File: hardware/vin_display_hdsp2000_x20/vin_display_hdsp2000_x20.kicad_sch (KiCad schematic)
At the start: 56 parts, among them J1 DEBUG, J2 USB_B_Micro, J3 DEBUG_UART, J4 IF_UART, J5 AUX_CONNECTOR, J6 Conn_01x02, Q1 BSS138, Q7 DMG2301L, SW1 SW_RESET, SW2 BOOTSEL, SW3 KNOB, U1 W25Q16JVSNIQ, U2 MIC23050-SYML, U3 RP2040, X1 12MHz

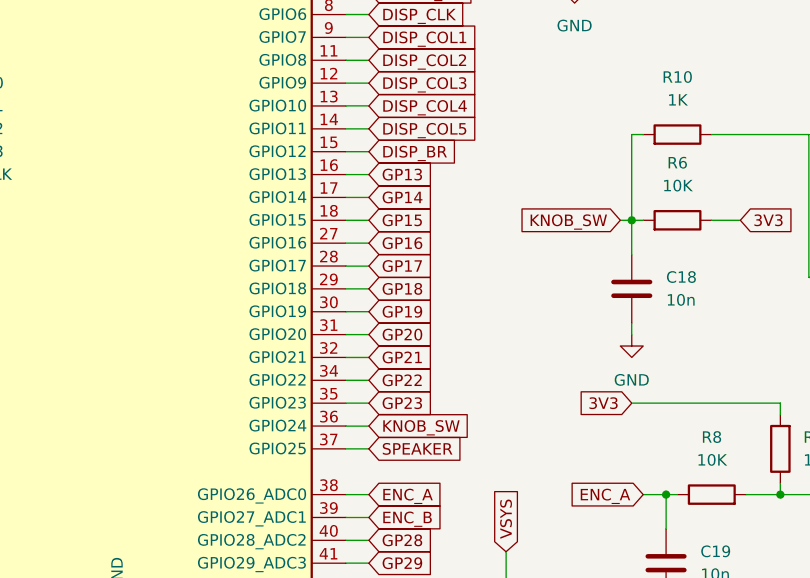
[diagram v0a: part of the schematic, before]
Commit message: hdsp2000_x20 minor changes
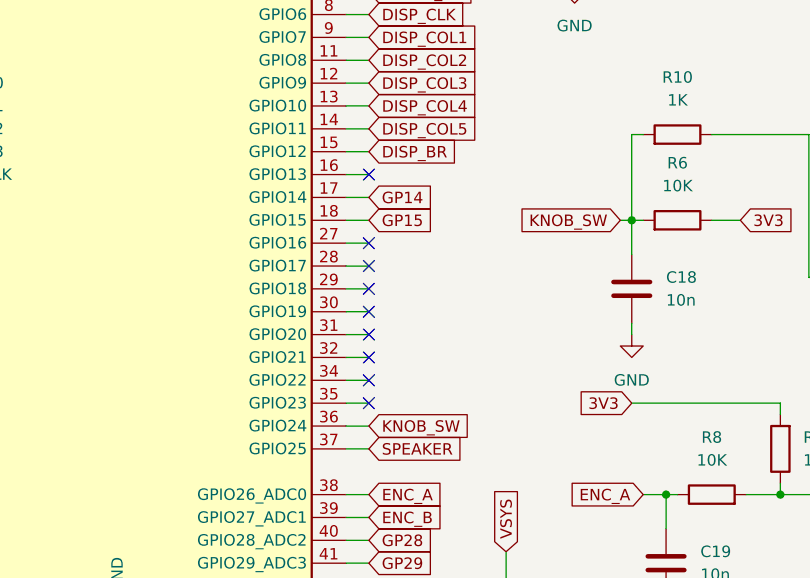
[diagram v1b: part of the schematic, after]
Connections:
- net GP13: no longer names the net of U3.16 (GPIO13)
- net GP16: no longer names the net of U3.27 (GPIO16)
- net GP17: no longer names the net of U3.28 (GPIO17)
- net GP18: no longer names the net of U3.29 (GPIO18)
- net GP19: no longer names the net of U3.30 (GPIO19)
- net GP20: no longer names the net of U3.31 (GPIO20)
- net GP21: no longer names the net of U3.32 (GPIO21)
- net GP22: no longer names the net of U3.34 (GPIO22)
- net GP23: no longer names the net of U3.35 (GPIO23)
- no-connect marks 1 -> 10
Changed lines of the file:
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@@
   (junction (at 130.81 22.86) (diameter 0) (color 0 0 0 0)
   )
+  (no_connect (at 181.61 97.79))
+  (no_connect (at 181.61 90.17))
+  (no_connect (at 181.61 92.71))
+  (no_connect (at 181.61 82.55))
+  (no_connect (at 181.61 95.25))
+  (no_connect (at 181.61 102.87))
+  (no_connect (at 181.61 107.95))
+  (no_connect (at 181.61 100.33))
+  (no_connect (at 181.61 105.41))
   (no_connect (at 49.53 176.53))
   (wire (pts (xy 125.73 80.01) (xy 128.27 80.01))
@@
     )
   )
-  (global_label "GP20" (shape input) (at 181.61 100.33 0) (fields_autoplaced)
-    (effects (font (size 1.27 1.27)) (justify left))
-    (property "Intersheetrefs" "${INTERSHEET_REFS}" (at 189.5542 100.33 0)
-      (effects (font (size 1.27 1.27)) (justify left) hide)
-    )
-  )
   (global_label "VSYS" (shape input) (at 100.33 152.4 180) (fields_autoplaced)
     (effects (font (size 1.27 1.27)) (justify right))
@@
     )
   )
-  (global_label "GP16" (shape input) (at 181.61 90.17 0) (fields_autoplaced)
-    (effects (font (size 1.27 1.27)) (justify left))
-    (property "Intersheetrefs" "${INTERSHEET_REFS}" (at 189.5542 90.17 0)
-      (effects (font (size 1.27 1.27)) (justify left) hide)
-    )
-  )
   (global_label "KNOB_SW" (shape input) (at 181.61 110.49 0) (fields_autoplaced)
     (effects (font (size 1.27 1.27)) (justify left))
@@
     )
   )
-  (global_label "GP13" (shape input) (at 181.61 82.55 0) (fields_autoplaced)
-    (effects (font (size 1.27 1.27)) (justify left))
-    (property "Intersheetrefs" "${INTERSHEET_REFS}" (at 189.5542 82.55 0)
-      (effects (font (size 1.27 1.27)) (justify left) hide)
-    )
-  )
   (global_label "GP28" (shape input) (at 181.61 123.19 0) (fields_autoplaced)
     (effects (font (size 1.27 1.27)) (justify left))
@@
     )
   )
-  (global_label "GP19" (shape input) (at 181.61 97.79 0) (fields_autoplaced)
-    (effects (font (size 1.27 1.27)) (justify left))
-    (property "Intersheetrefs" "${INTERSHEET_REFS}" (at 189.5542 97.79 0)
-      (effects (font (size 1.27 1.27)) (justify left) hide)
-    )
-  )
   (global_label "UART1_TX" (shape input) (at 60.96 137.16 180) (fields_autoplaced)
     (effects (font (size 1.27 1.27)) (justify right))
@@
     )
   )
-  (global_label "GP22" (shape input) (at 181.61 105.41 0) (fields_autoplaced)
-    (effects (font (size 1.27 1.27)) (justify left))
-    (property "Intersheetrefs" "${INTERSHEET_REFS}" (at 189.5542 105.41 0)
-      (effects (font (size 1.27 1.27)) (justify left) hide)
-    )
-  )
   (global_label "GP14" (shape input) (at 181.61 85.09 0) (fields_autoplaced)
     (effects (font (size 1.27 1.27)) (justify left))
@@
     (effects (font (size 1.27 1.27)) (justify left))
     (property "Intersheetrefs" "${INTERSHEET_REFS}" (at 79.9306 155.5507 90)
-      (effects (font (size 1.27 1.27)) (justify left) hide)
-    )
-  )
-  (global_label "GP17" (shape input) (at 181.61 92.71 0) (fields_autoplaced)
-    (effects (font (size 1.27 1.27)) (justify left))
-    (property "Intersheetrefs" "${INTERSHEET_REFS}" (at 189.5542 92.71 0)
       (effects (font (size 1.27 1.27)) (justify left) hide)
     )
@@
     )
   )
-  (global_label "GP23" (shape input) (at 181.61 107.95 0) (fields_autoplaced)
-    (effects (font (size 1.27 1.27)) (justify left))
-    (property "Intersheetrefs" "${INTERSHEET_REFS}" (at 189.5542 107.95 0)
-      (effects (font (size 1.27 1.27)) (justify left) hide)
-    )
-  )
   (global_label "DISP_COL1" (shape input) (at 181.61 67.31 0) (fields_autoplaced)
     (effects (font (size 1.27 1.27)) (justify left))
@@
     )
   )
-  (global_label "GP21" (shape input) (at 181.61 102.87 0) (fields_autoplaced)
-    (effects (font (size 1.27 1.27)) (justify left))
-    (property "Intersheetrefs" "${INTERSHEET_REFS}" (at 189.5542 102.87 0)
-      (effects (font (size 1.27 1.27)) (justify left) hide)
-    )
-  )
   (global_label "SPEAKER" (shape input) (at 181.61 146.05 180) (fields_autoplaced)
     (effects (font (size 1.27 1.27)) (justify right))
@@
       (effects (font (size 1.27 1.27)) (justify left) hide)
     )
-  )
-  (global_label "GP18" (shape input) (at 181.61 95.25 0) (fields_autoplaced)
-    (effects (font (size 1.27 1.27)) (justify left))
-    (property "Intersheetrefs" "${INTERSHEET_REFS}" (at 189.5542 95.25 0)
-      (effects (font (size 1.27 1.27)) (justify left) hide)
-    )
